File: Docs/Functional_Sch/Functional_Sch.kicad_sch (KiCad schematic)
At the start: 53 parts

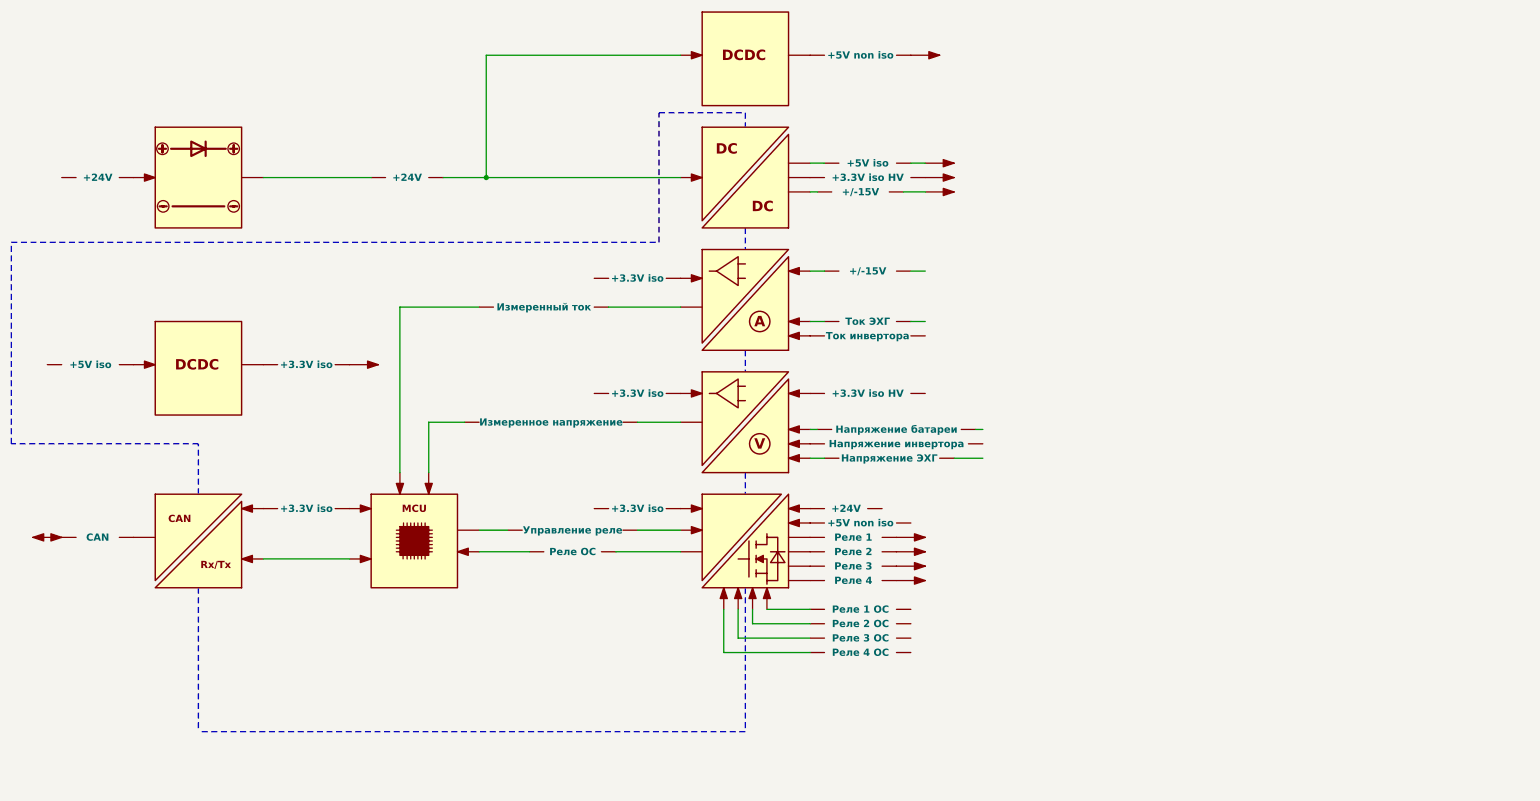
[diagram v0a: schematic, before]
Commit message: VER1.0: плата разведена, файлы по плате готовы
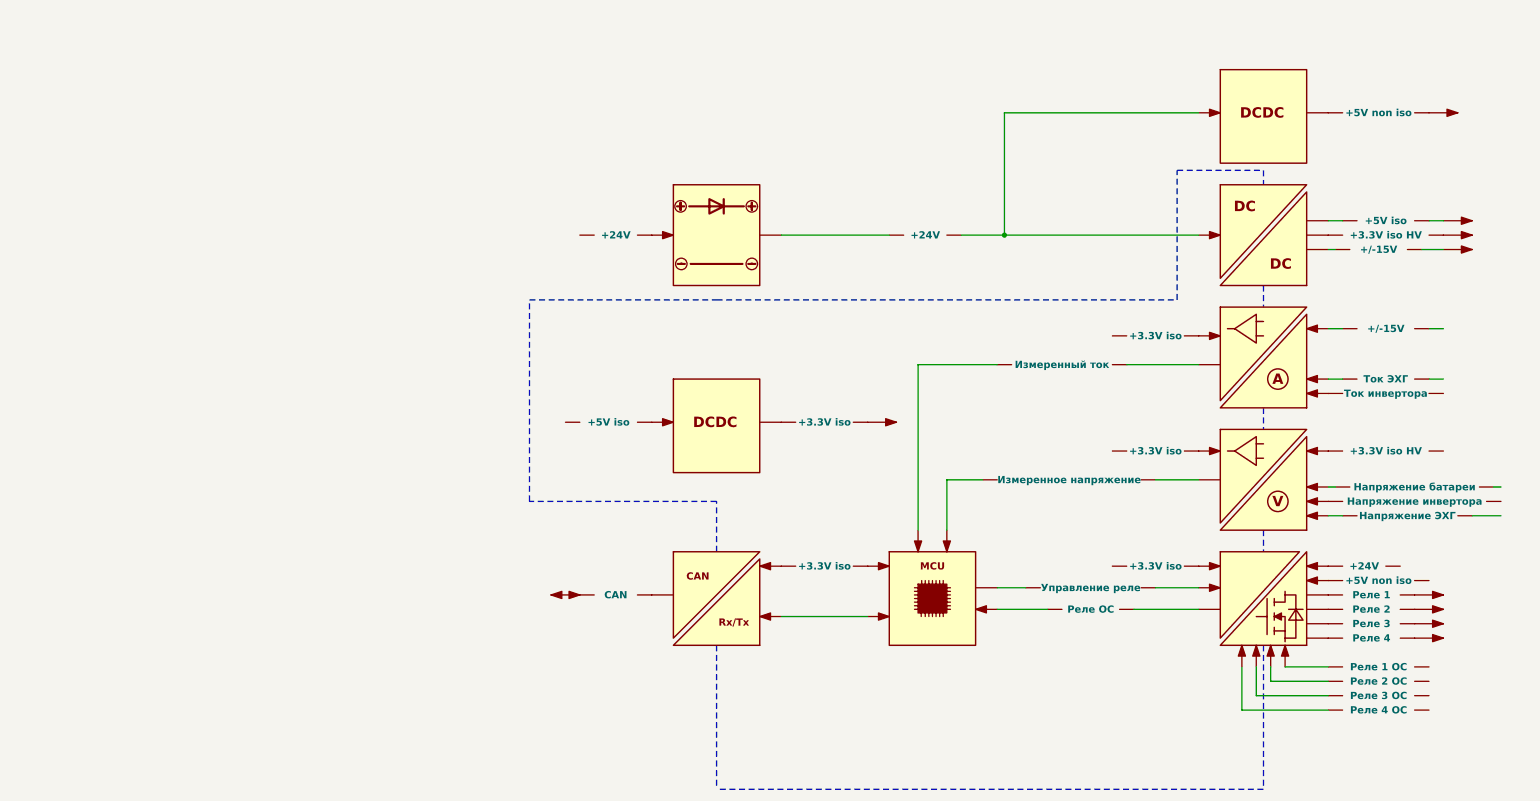
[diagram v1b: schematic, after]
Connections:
- net at D2.: now also D12.; no longer D11.
- net at D43.: now also D44.; no longer D2.
- net at D12.: now also D13.; no longer D2.
- net at D57.: now also D6.; no longer D4.
- net at D6.: now also D35.; no longer D57.
- net at D30.: now also D34.
- net at D34.: now also D41.; no longer D30.
- net at D54.: now also D5.; no longer D4.
- net at D5.: now also D20.; no longer D54.
- net at D56.: now also D5.
- net at D52.: now also D34.; no longer D4.
- net at D55.: now also D34.
- net at D4.: now also D51.; no longer D6.
- net at D53.: now also D5.; no longer D4.
- net at D51.: now also D7.; no longer D4.
- net at D32.: now also D7.
- net at D7.: now also D45.; no longer D32.
- net at D27.: now also D5.
- net at D29.: now also D34.
- net at D40.: now also D5.
- net at D31.: now also D34.
- net at D9.: now also D1.
- net at D1.: now also D10.; no longer D9.
- net at D26.: now also D5.
- net at D35.: now also D36.; no longer D6.
- net at D28.: now also D37.
- net at D25.: no longer D5.
- net at D42.: no longer D5.
- net at D24.: no longer D5.
- net at D41.: no longer D34.
- net at D33.: now also D7.
- net at D48.: no longer D7.
- net at D45.: no longer D7.
- new net: D11., D2.
- new net: D10., D2., D3.
- new net: D2., D43.
- new net: D4., D57.
- new net: D4., D54.
- new net: D4., D52.
- new net: D4., D6.
- new net: D4., D53.
- new net: D25., D5.
- new net: D42., D5.
- new net: D24., D5.
- new net: D48., D7.
